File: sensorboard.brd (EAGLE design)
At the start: 95.5 x 64 mm, 20 parts, among them IC1 LD117AS18TR, K2 JTN-PCB-DC18V, Q1 BC639, Q2 BC639

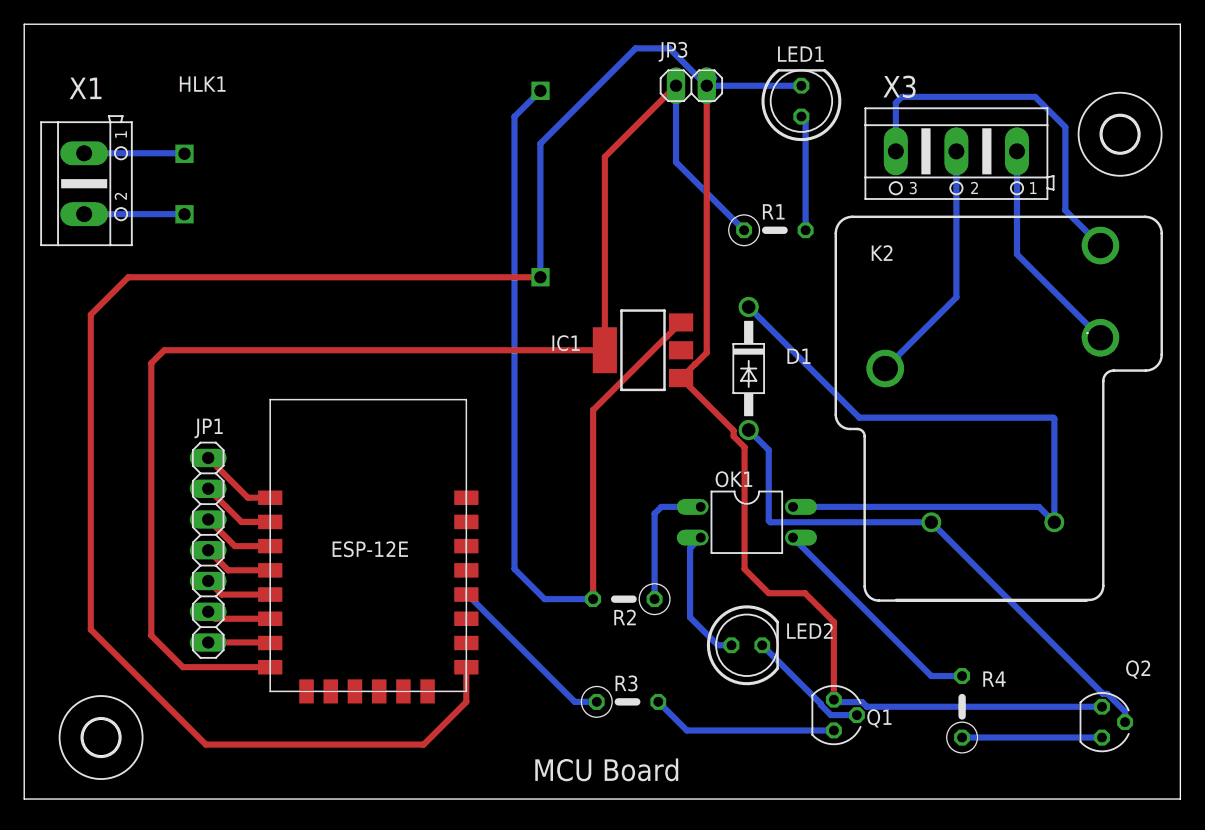
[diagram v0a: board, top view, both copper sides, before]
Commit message: Add files via upload
Version2 (88 X 59.50)
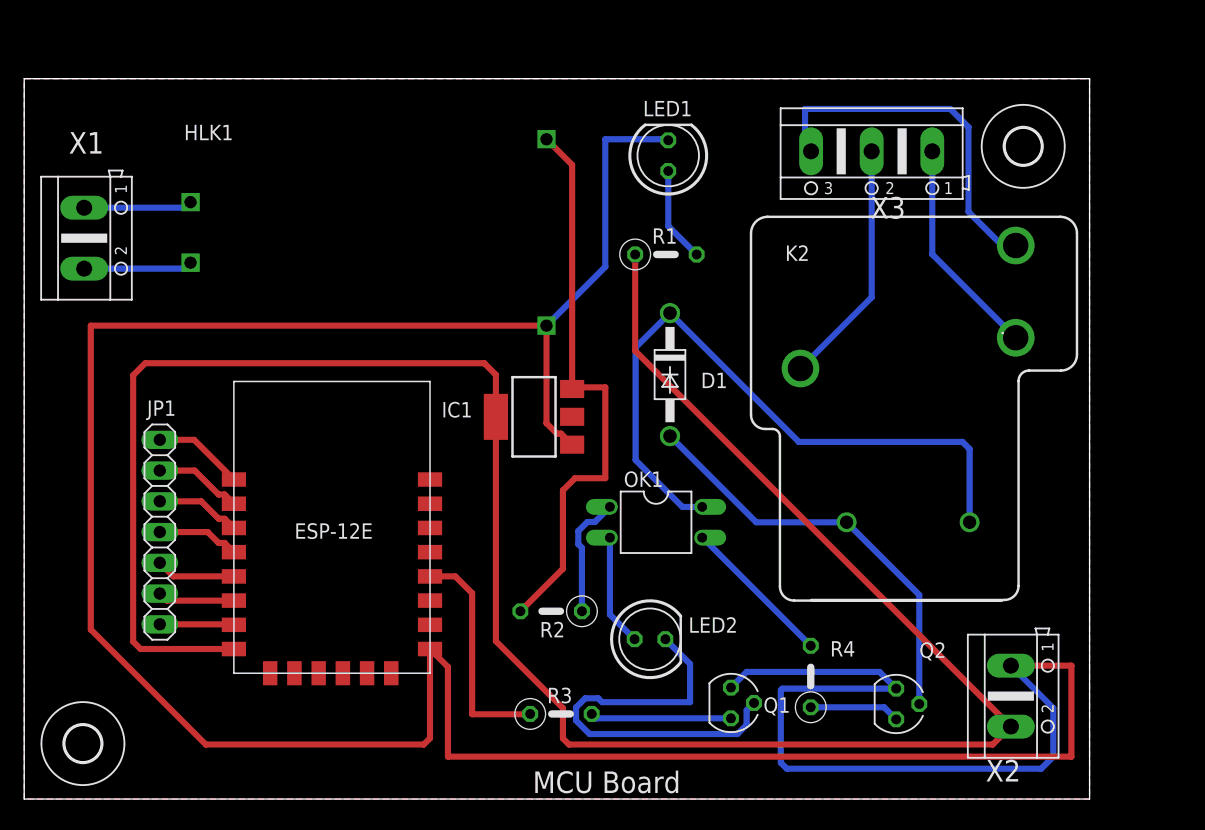
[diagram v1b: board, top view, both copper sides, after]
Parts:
- removed JP3: (no value), pinhead:1X02
- added X2: (no value), con-ptr500:AK500/2
- moved Q2 17.1 mm to (72.0, 7.85)
- moved R4 12.7 mm to (65.0, 10.1)
- moved LED1 11.9 mm to (53.2, 53.1)
- moved IC1 10.5 mm to (42.1, 31.6)
- moved R1 9.22 mm to (53.0, 45.0)
- moved Q1 8.56 mm to (58.4, 7.93)
- moved H1 8.06 mm to (82.5, 53.9)
- moved LED2 8.02 mm to (51.7, 13.2)
- moved OK1 7.50 mm to (52.2, 22.9)
- moved K2 7.00 mm to (73.0, 22.9)
- moved X3 7.00 mm to (70.0, 53.5)
- moved D1 6.52 mm to (53.3, 35.1)
- moved R2 6.08 mm to (43.5, 15.5)
- moved R3 5.59 mm to (44.3, 7.03)
- moved X1 4.50 mm to (4.95, 46.3)
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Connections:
- net GND: now also X2.1; no longer JP3.2
- net VDD3V3: now also X2.2; no longer JP3.1
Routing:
- net VDD3V3: track 109.9 -> 183.3 mm
- net GND: track 222.7 -> 271.8 mm
- net 5V: track 73.8 -> 47.2 mm
- net N$6: track 10.3 -> 33.9 mm
- net N$11: track 45.0 -> 35.0 mm
- net N$8: track 18.7 -> 12.7 mm
- net REL1: track 14.5 -> 18.9 mm
- net N$9: track 11.6 -> 7.47 mm
- net N$10: track 59.7 -> 55.9 mm
- net N$7: track 15.5 -> 11.7 mm
- net N$5: track 11.3 -> 9.23 mm
- net N$3: track 9.54 -> 7.87 mm
- net NRST: track 6.48 -> 7.48 mm
- net GPIO14: track 5.58 -> 6.58 mm
- net GPIO13: track 5.14 -> 6.14 mm
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- added copper zone on layer 1, net GND
- added copper zone on layer 16, net GND
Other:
- board size 95.5 x 64 mm -> 88 x 59.5 mm
